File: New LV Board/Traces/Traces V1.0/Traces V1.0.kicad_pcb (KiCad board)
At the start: 2 copper layers, 103.1 x 54.3 mm, 13 parts, among them J1 B15B-PH-K-S, J2 B15B-PH-K-S, J3 B15B-PH-K-S, J4 Conn_01x12, J6 Conn_01x12, J7 Conn_01x12

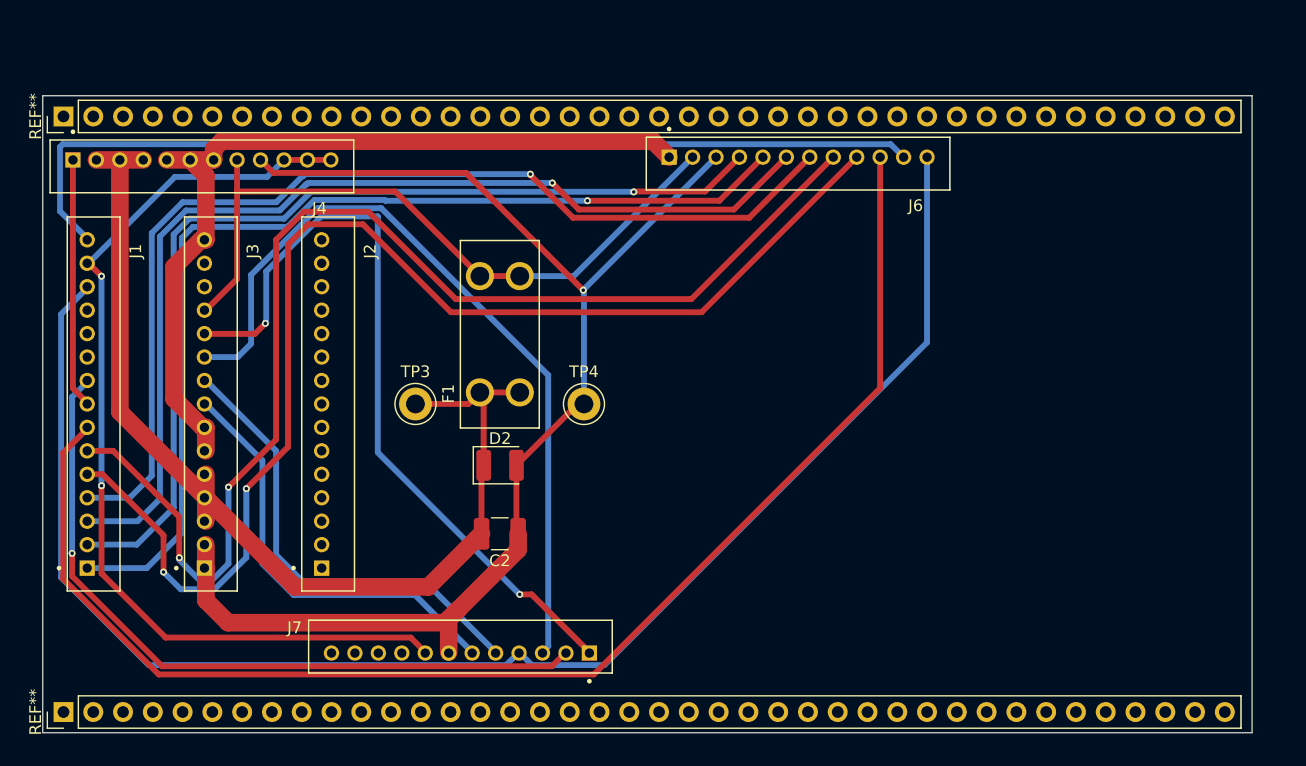
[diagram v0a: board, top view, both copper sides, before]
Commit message: No significant changes just random kicad BS
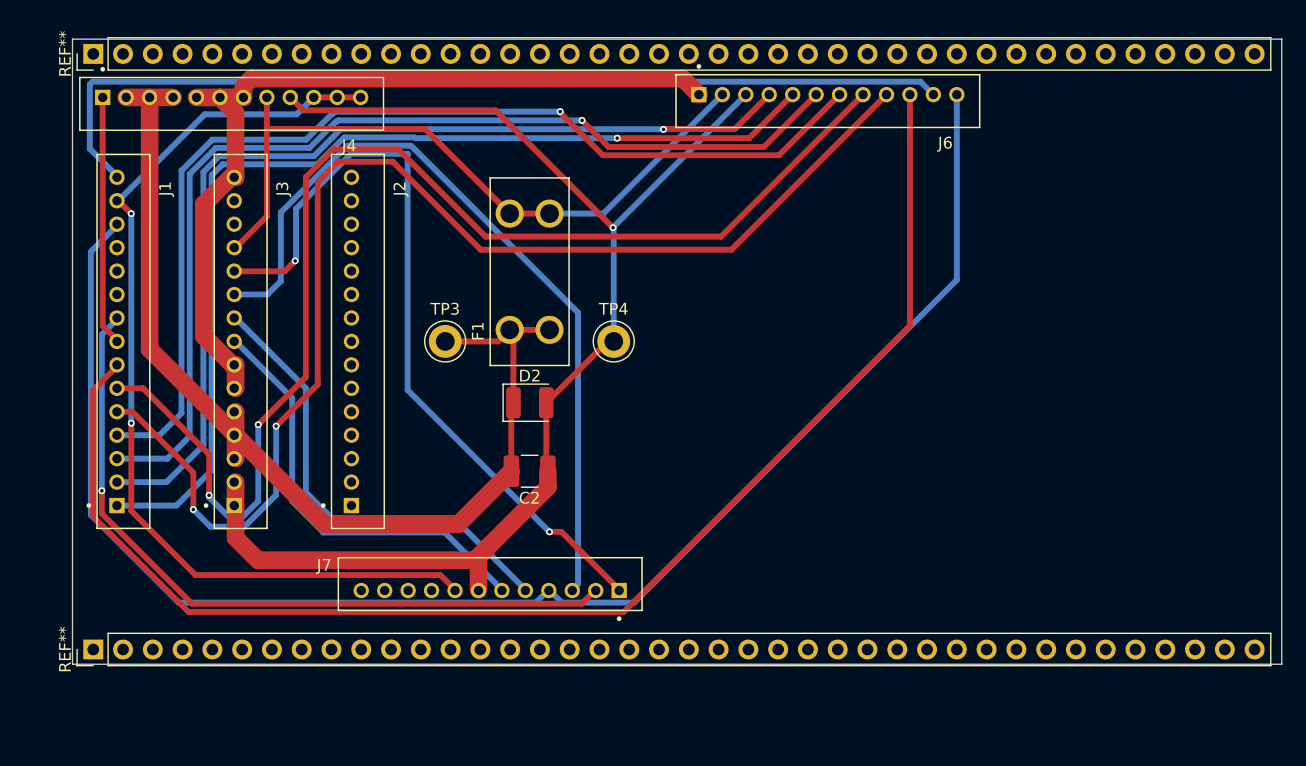
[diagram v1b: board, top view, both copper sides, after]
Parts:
- moved D2 5.91 mm to (85.5, 121.2)
- moved F1 5.91 mm to (85.5, 110.0)
- moved J6 5.91 mm to (110.9, 95.5)
- moved J7 5.91 mm to (82.1, 136.7)
- moved REF** 5.91 mm to (48.3, 142.2)
- moved REF** 5.91 mm to (48.3, 91.4)
- moved C2 5.91 mm to (85.5, 127.0)
- moved J2 5.91 mm to (70.8, 116.0)
- moved TP4 5.91 mm to (92.7, 116.0)
- moved J1 5.91 mm to (50.8, 116.0)
- moved J3 5.91 mm to (60.8, 116.0)
- moved J4 5.91 mm to (60.1, 95.7)
- moved TP3 5.91 mm to (78.3, 116.0)
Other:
- board size 103.1 x 54.3 mm -> 103.1 x 53.3 mm
